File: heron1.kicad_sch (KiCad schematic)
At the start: 9 parts, among them SW1 SW_Push, U1 DRV8835

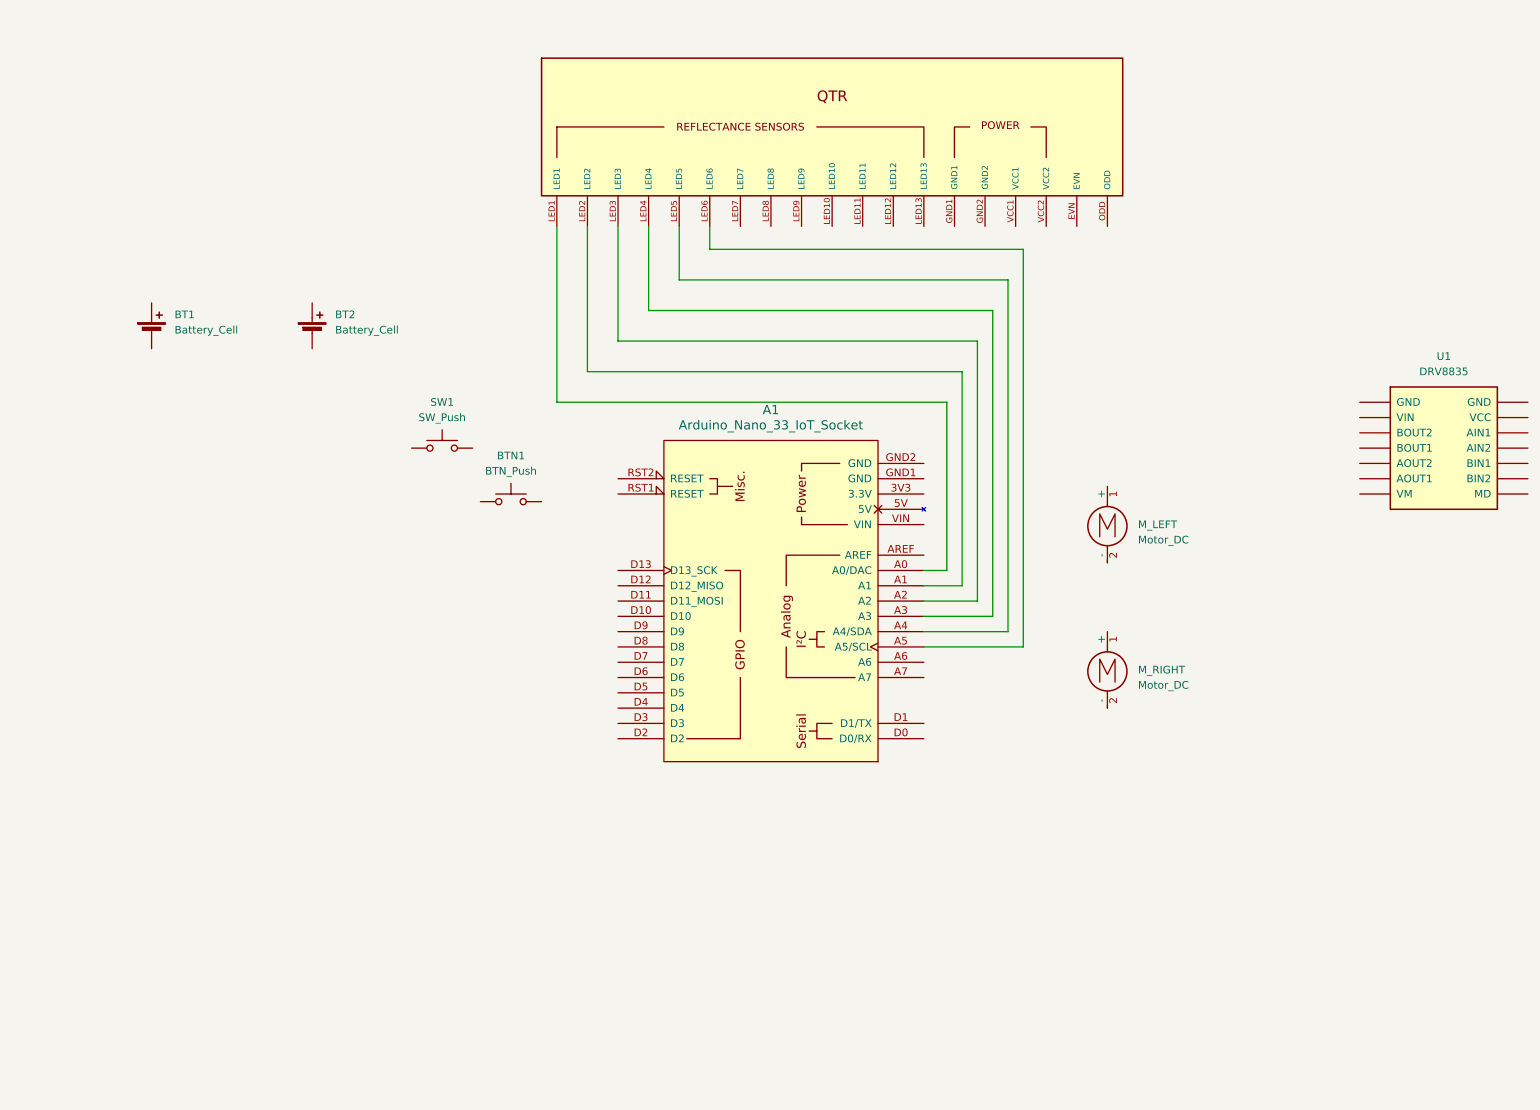
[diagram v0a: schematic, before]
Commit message: first stage of schematic complete
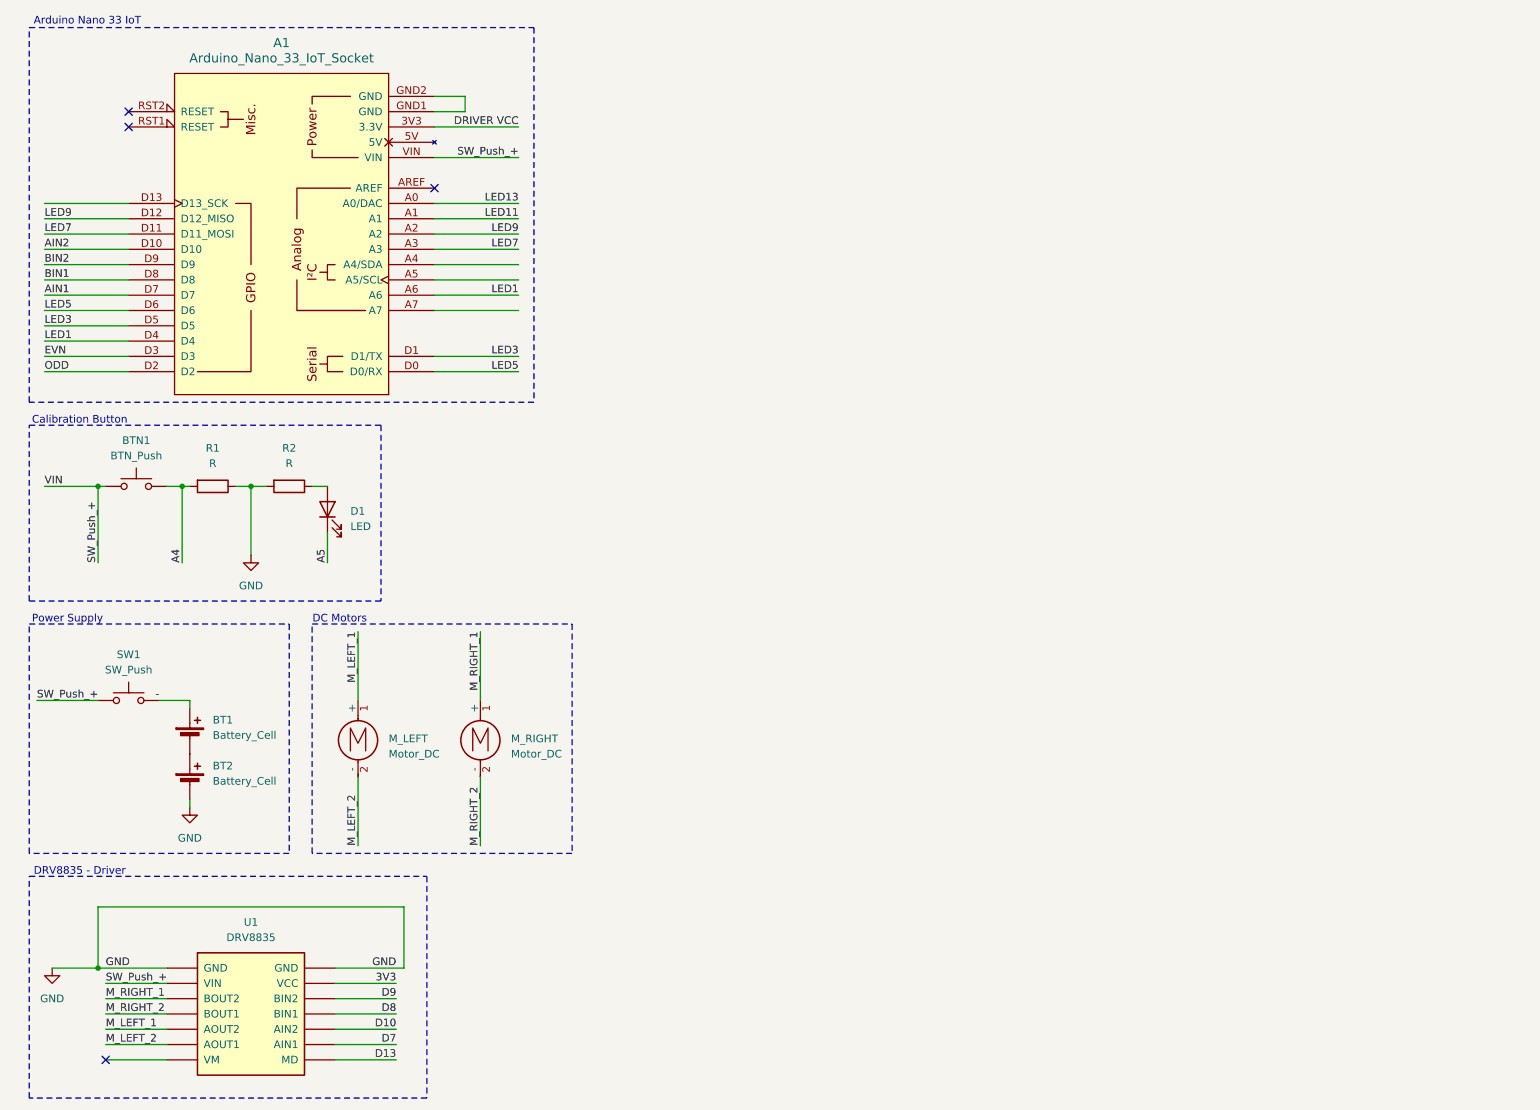
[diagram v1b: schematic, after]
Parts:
- removed ?: ~, QTR-8A:QTR-8A, symbol QTR-8A:QTR-8A
- added D1: LED, symbol Device:LED
- added R1, R2: R, symbol Device:R
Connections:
- net -: now reaches BT1.1 (+)
- net -: now also SW1.2
- net at BT1.2 (-): now also BT2.1 (+)
- net SW_Push_+: now reaches BTN1.1
- net SW_Push_+: now also A1.VIN, SW1.1, U1. (VM)
- net A4: now reaches BTN1.2
- net A4: now also R1.2
- net M_LEFT_1: now reaches M_LEFT.1 (+)
- net M_LEFT_1: now also U1. (VM)
- net M_LEFT_2: now reaches M_LEFT.2 (-)
- net M_LEFT_2: now also U1. (VM)
- net LED13: now reaches A1.A0 (A0/DAC)
- net LED11: now reaches A1.A1
- net LED9: now reaches A1.A2
- net LED9: now also A1.D12 (D12_MISO)
- net LED7: now reaches A1.A3
- net LED7: now also A1.D11 (D11_MOSI)
- net M_RIGHT_1: now reaches M_RIGHT.1 (+)
- net M_RIGHT_1: now also U1. (VM)
- net M_RIGHT_2: now reaches M_RIGHT.2 (-)
- net M_RIGHT_2: now also U1. (VM)
- net DRIVER VCC: now reaches A1.3V3 (3.3V)
- net LED1: now reaches A1.A6
- net LED1: now also A1.D4
- net LED5: now reaches A1.D0 (D0/RX)
- net LED5: now also A1.D6
- net LED3: now reaches A1.D1 (D1/TX)
- net LED3: now also A1.D5
- net AIN2: now reaches A1.D10
- net ODD: now reaches A1.D2
- net EVN: now reaches A1.D3
- net AIN1: now reaches A1.D7
- net BIN1: now reaches A1.D8
- net BIN2: now reaches A1.D9
- net at A1.GND1 (GND): now also A1.GND2 (GND)
- net GND: now reaches BT2.2 (-)
- net GND: now also U1. (VM), R1.1, R2.2
- new net: D1.2 (A), R2.1
- new net 3V3: U1. (VM)
- new net A5: D1.1 (K)
- new net D10: U1. (VM)
- new net D13: U1. (VM)
- new net D7: U1. (VM)
- new net D8: U1. (VM)
- new net D9: U1. (VM)
- no-connect marks 0 -> 4
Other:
- note added: "Arduino Nano 33 IoT"
- note added: "Calibration Button"
- note added: "DC Motors"
- note added: "DRV8835 - Driver"
- note added: "Power Supply"
- moved on the sheet: A1, BT1, BT2, BTN1, M_LEFT, M_RIGHT, SW1, U1
